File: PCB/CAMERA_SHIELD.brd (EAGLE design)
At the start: 79.7 x 100.3 mm, 73 parts, among them IC4 LSF0204PWR, J1 47346-0001, Q1 FDN304P, Q2 FDN304P, Q3 SSM3J338R,LF, Q4 SSM3J338R,LF, Q5 FDN304P, U1 LARA-R2

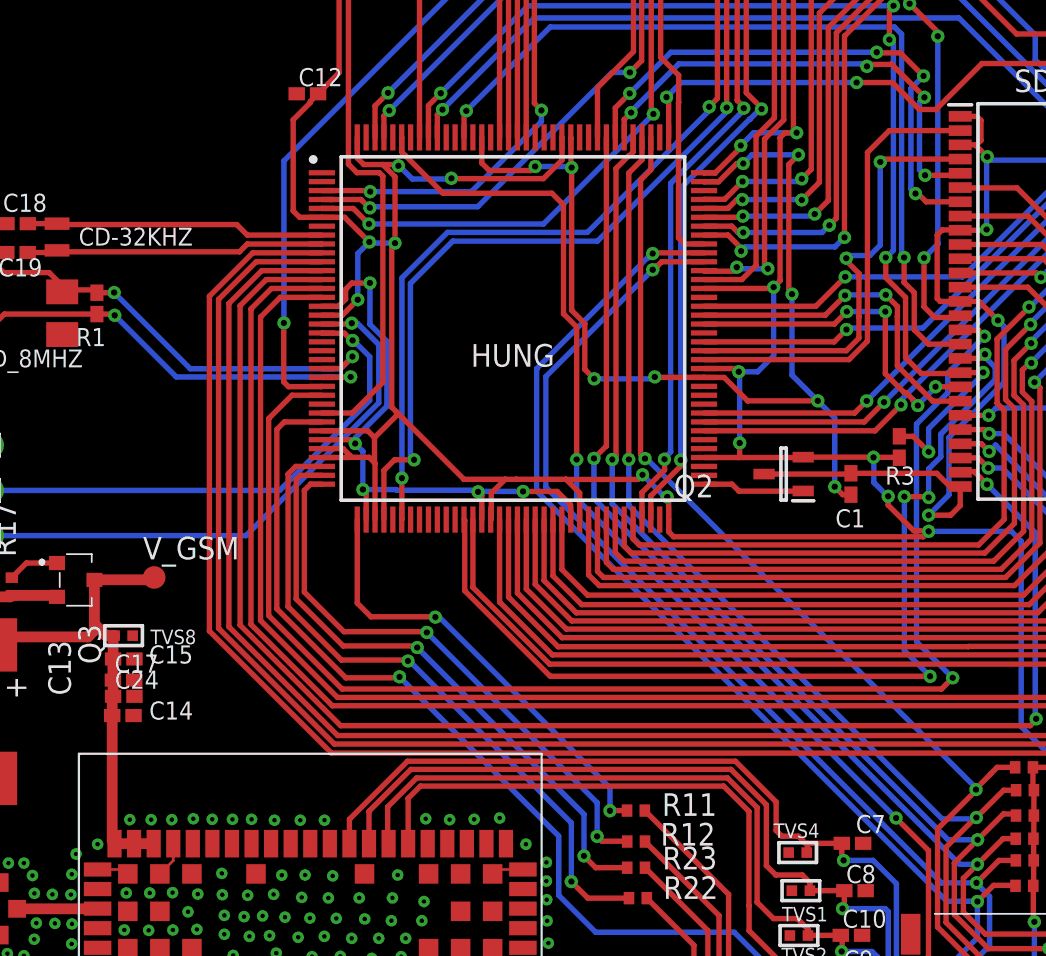
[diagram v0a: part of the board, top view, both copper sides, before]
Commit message: fix router
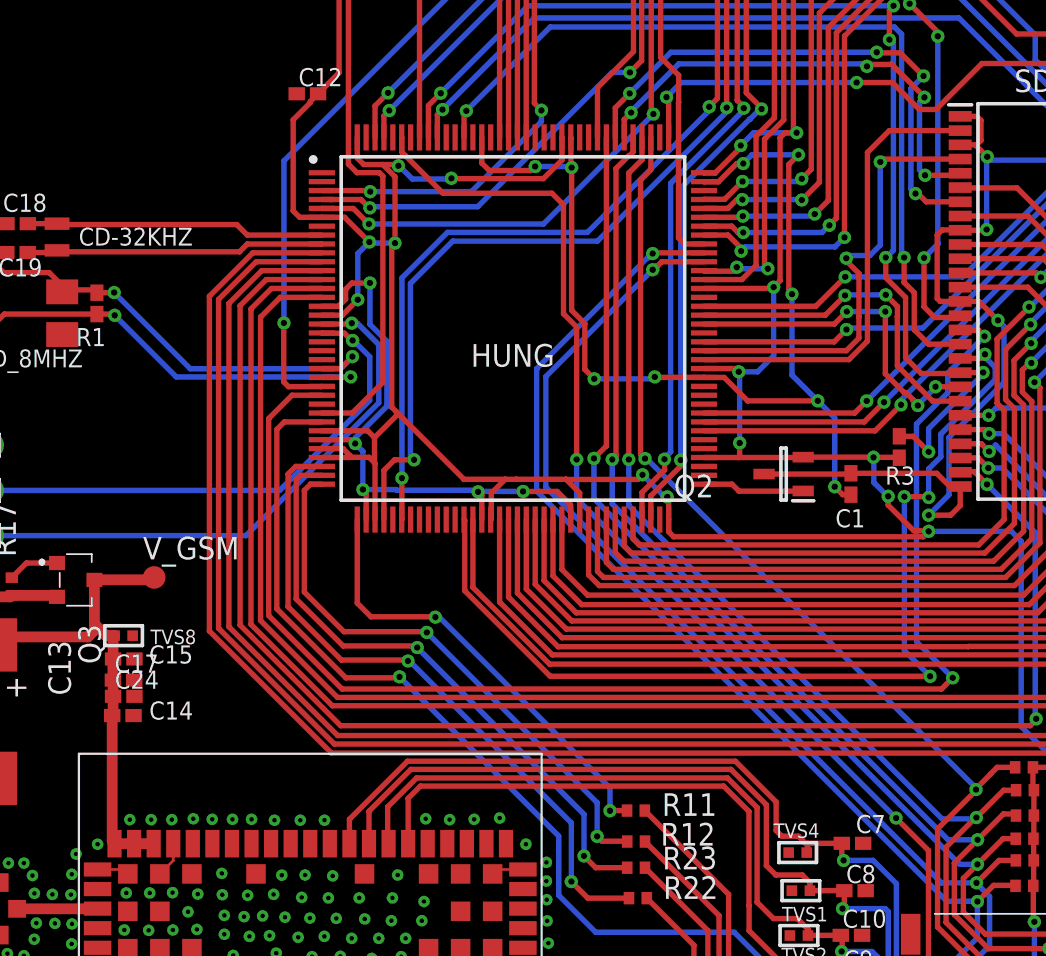
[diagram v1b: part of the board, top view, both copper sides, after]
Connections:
- removed net N$196: U1.51, U1.52, U1.53
- net V_GSM: now also U1.51, U1.52, U1.53
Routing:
- net V_GSM: track 25.2 -> 27.6 mm
- net N$196: track 2.20 -> 0.00 mm
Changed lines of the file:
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@@
 <wire x1="54.873" y1="67.1612" x2="56.8828875" y2="67.1612" width="0.3048" layer="1"/>
 <wire x1="72.12" y1="71.1" x2="72.12" y2="71.11" width="0.3048" layer="1"/>
-<wire x1="59.37" y1="65.61" x2="59.333" y2="65.647" width="0.3048" layer="1"/>
 <wire x1="58.3970875" y1="65.647" x2="59.333" y2="65.647" width="0.3048" layer="1"/>
 <wire x1="56.8828875" y1="67.1612" x2="58.3970875" y2="65.647" width="0.3048" layer="1"/>
@@
 <contactref element="V_GSM" pad="TP"/>
 <contactref element="TVS8" pad="2"/>
+<contactref element="U1" pad="52"/>
+<contactref element="U1" pad="53"/>
+<contactref element="U1" pad="51"/>
 <contactref element="Q3" pad="3"/>
 <wire x1="15.4" y1="39.35" x2="15.27" y2="39.22" width="0.6096" layer="1"/>
@@
 <wire x1="13.09" y1="32.67" x2="13.09" y2="33.57" width="0.6096" layer="1"/>
 <wire x1="13.09" y1="33.57" x2="13.08" y2="33.58" width="0.6096" layer="1"/>
+<wire x1="14.27" y1="24.39" x2="15.37" y2="24.39" width="0.6096" layer="1"/>
+<wire x1="13.17" y1="24.39" x2="14.27" y2="24.39" width="0.6096" layer="1"/>
 <wire x1="13.04" y1="31.59" x2="13.04" y2="24.52" width="0.6096" layer="1"/>
-<wire x1="13.04" y1="31.59" x2="13.04" y2="32.62" width="0.6096" layer="1"/>
-<wire x1="13.04" y1="32.62" x2="13.09" y2="32.67" width="0.6096" layer="1"/>
+<wire x1="13.04" y1="24.52" x2="13.17" y2="24.39" width="0.6096" layer="1"/>
+<wire x1="13.09" y1="32.67" x2="13.09" y2="31.64" width="0.6096" layer="1"/>
+<wire x1="13.09" y1="31.64" x2="13.04" y2="31.59" width="0.6096" layer="1"/>
 </signal>
 <signal name="USART2_CTS">
@@
 <via x="10.62" y="13.79" extent="1-16" drill="0.25"/>
 </signal>
-<signal name="N$196">
-<contactref element="U1" pad="52"/>
-<contactref element="U1" pad="53"/>
-<contactref element="U1" pad="51"/>
-<wire x1="14.27" y1="24.39" x2="15.37" y2="24.39" width="0.6096" layer="1"/>
-<wire x1="13.17" y1="24.39" x2="14.27" y2="24.39" width="0.6096" layer="1"/>
-</signal>
 </signals>
